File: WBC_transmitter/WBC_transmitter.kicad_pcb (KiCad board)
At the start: 2 copper layers, 153.7 x 88.9 mm, 91 parts, among them J1 Conn_01x03_Female, J2 Conn_01x02_Female, J3 Conn_01x05_Male, J4 Conn_01x03_Female, J5 Conn_01x03_Female, J6 Conn_01x01_Male, J7 Conn_01x01_Male, Q1 IRF740, Q2 IRF740, Q3 IRF740, Q4 IRF740, Q5 IRF740, Q6 IRF740, U1 IR2110, U2 IR2110, U3 IR2110, U4 PIC16F1933-I_SS, U5 TL082, Y1 Crystal

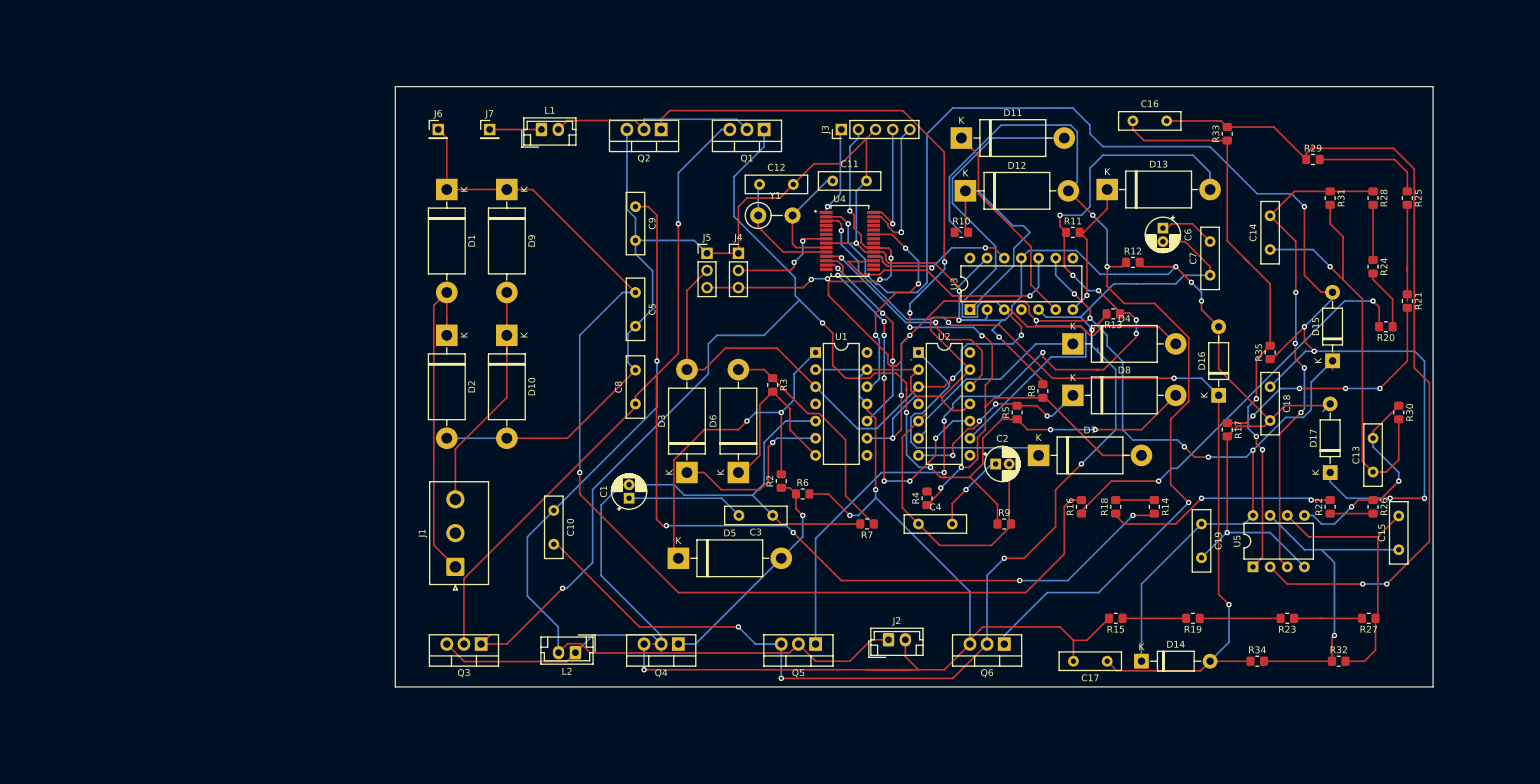
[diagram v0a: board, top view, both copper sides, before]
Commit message: Routing done
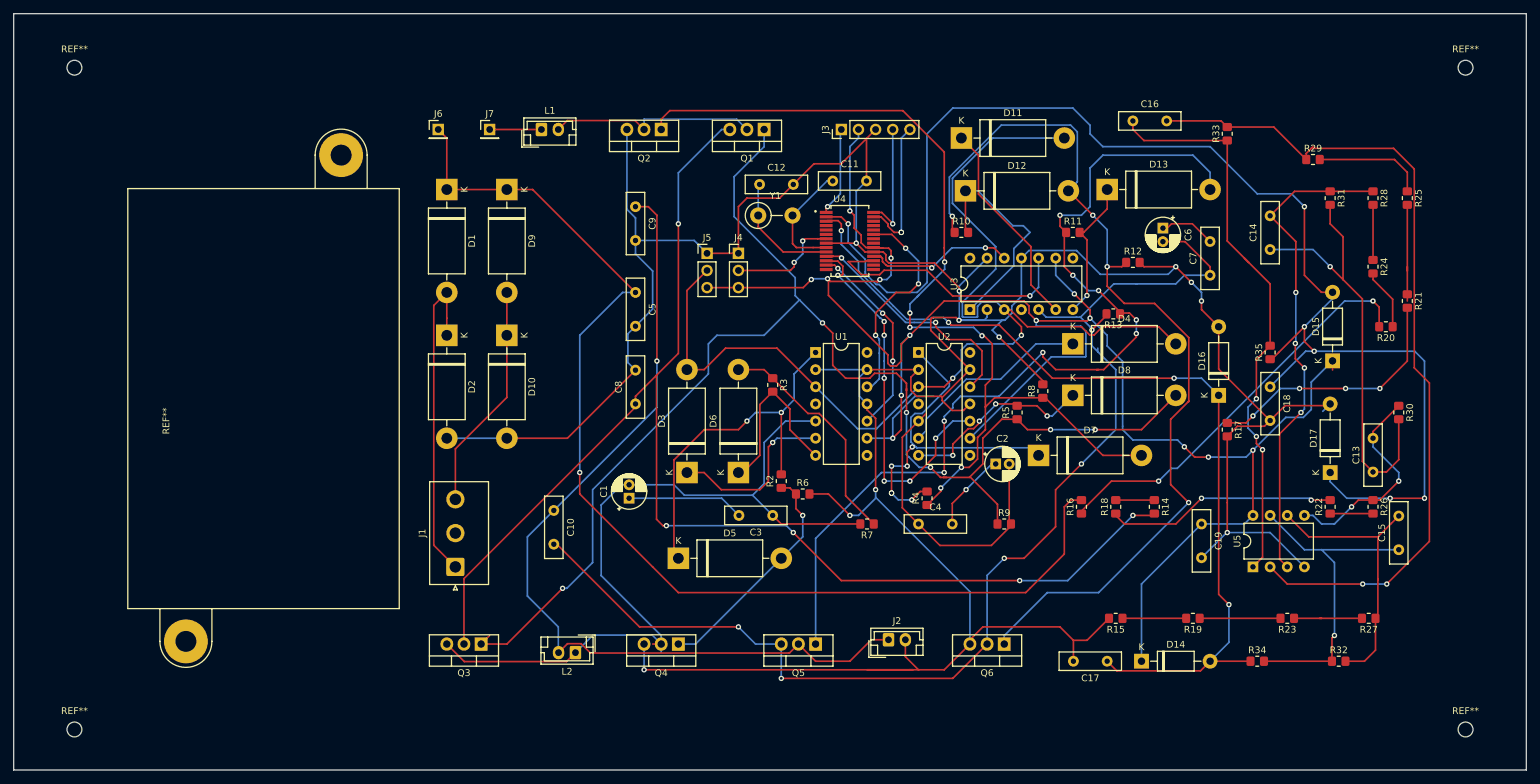
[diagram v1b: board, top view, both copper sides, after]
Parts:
- added REF**: MountingHole_2.2mm_M2_ISO7380, MountingHole:MountingHole_2.2mm_M2_ISO7380, F.Cu at (255.0, 48.0)
- added REF**: MountingHole_2.2mm_M2_ISO7380, MountingHole:MountingHole_2.2mm_M2_ISO7380, F.Cu at (49.0, 48.0)
- added REF**: MountingHole_2.2mm_M2_ISO7380, MountingHole:MountingHole_2.2mm_M2_ISO7380, F.Cu at (255.0, 146.0)
- added REF**: MountingHole_2.2mm_M2_ISO7380, MountingHole:MountingHole_2.2mm_M2_ISO7380, F.Cu at (49.0, 146.0)
- added REF**: Heatsink_62x40mm_2xFixation3mm, Heatsink:Heatsink_62x40mm_2xFixation3mm, F.Cu at (97.0, 128.0)
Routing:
- net Net-(D7-Pad1): track 39.3 -> 55.6 mm, vias 0 -> 6
- net INV-L: track 139.5 -> 139.0 mm, vias 3 -> 4
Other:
- board size 153.7 x 88.9 mm -> 224 x 112 mm
